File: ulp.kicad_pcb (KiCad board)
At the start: 2 copper layers, 102 x 82.6 mm, 49 parts, among them J1 Conn_01x01_Pin, J2 Conn_01x01_Pin, SW1 SW_Push_45deg, SW10 SW_Push_45deg, SW11 SW_Push_45deg, SW12 SW_Push_45deg, SW13 SW_Push_45deg, SW14 SW_Push_45deg, SW15 SW_Push_45deg, SW16 SW_Push_45deg, SW17 SW_Push_45deg, SW18 SW_Push_45deg, SW19 SW_SPDT, SW2 SW_Push_45deg, SW20 SW_Push_Dual, SW3 SW_Push_45deg, SW4 SW_Push_45deg, SW5 SW_Push_45deg, SW6 SW_Push_45deg, SW7 SW_Push_45deg, SW8 SW_Push_45deg, SW9 SW_Push_45deg, U2 XIAO-nRF52840-SMD

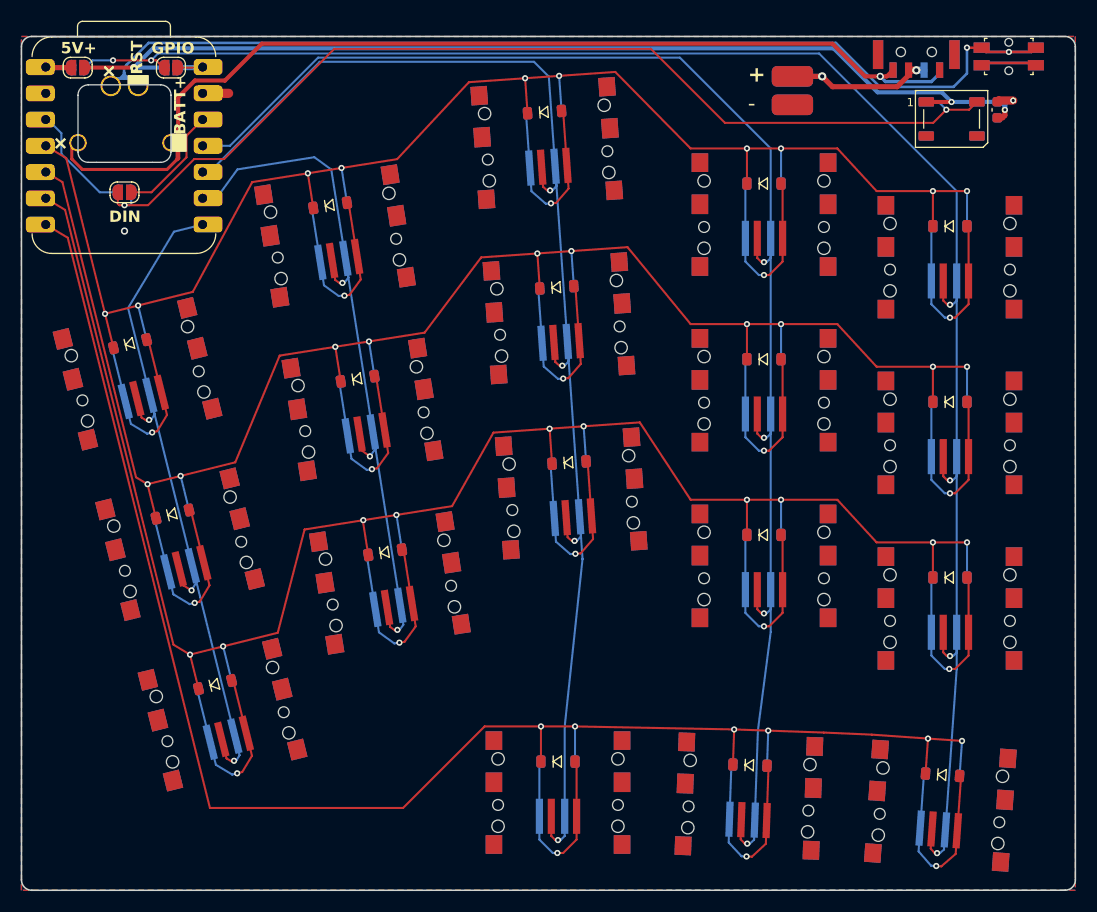
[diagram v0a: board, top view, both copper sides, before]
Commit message: add new pcb stuff
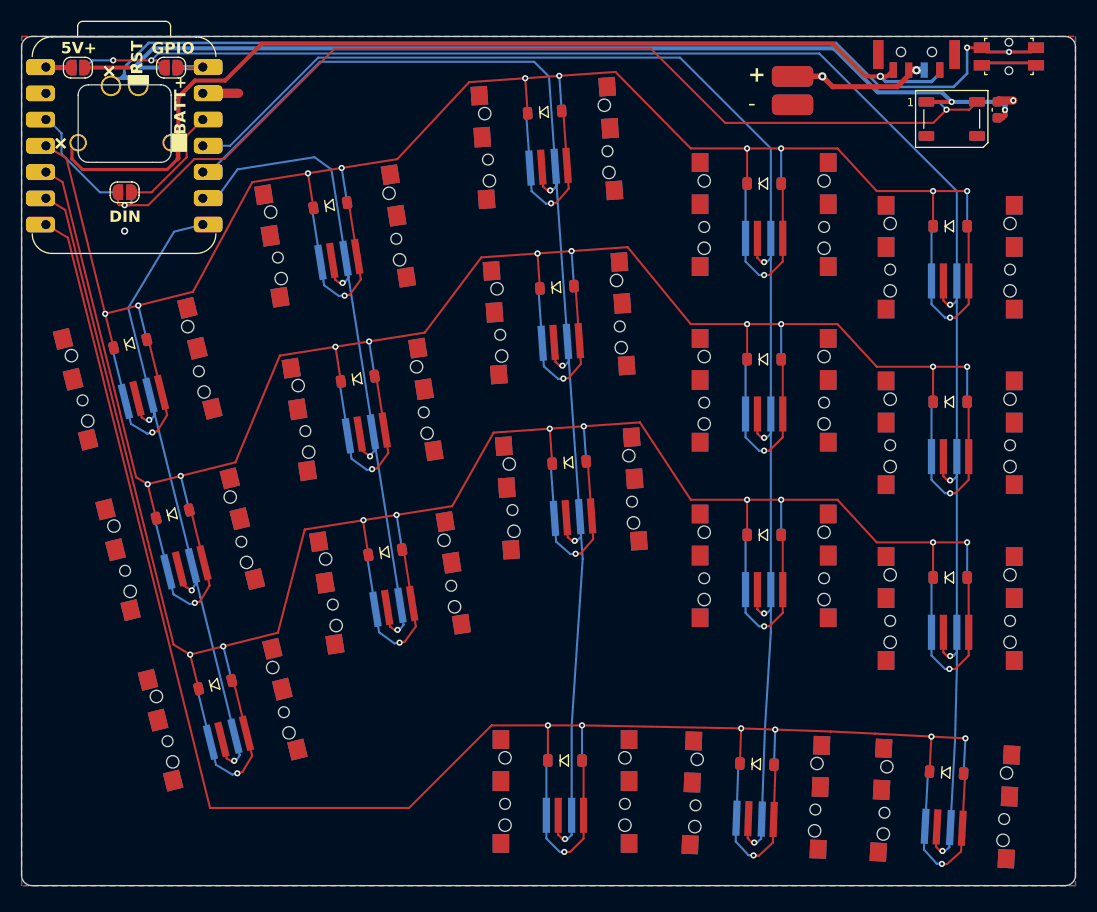
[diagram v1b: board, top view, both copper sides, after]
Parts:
- moved SW17 0.68 mm to (169.7, 128.2)
- moved D17 0.68 mm to (169.8, 125.2)
- moved SW16 0.68 mm to (151.2, 127.8)
- moved D16 0.68 mm to (151.2, 124.8)
- moved SW18 0.49 mm to (188.0, 129.0), turned to -3 degrees
- moved D18 0.45 mm to (188.2, 126.0), turned to -3 degrees
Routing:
- net GND: track 15.0 -> 15.9 mm
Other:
- board size 102 x 82.6 mm -> 102 x 82.2 mm
